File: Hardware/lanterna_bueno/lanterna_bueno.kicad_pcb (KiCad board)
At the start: 2 copper layers, 78.8 x 56.5 mm, 62 parts, among them J1 Conn_01x02_Male, J10 Conn_01x03_Male, J11 Conn_01x03_Male, J2 Conn_01x02_Male, J3 Conn_01x02_Male, J4 Conn_01x03_Male, J5 Conn_01x03_Male, J6 Conn_01x03_Male, J7 Conn_01x03_Male, J8 Conn_01x03_Male, J9 Conn_01x03_Male, P1 USB_C_Plug_USB2.0, Q1 BC807, Q2 2SK4075, Q3 2SK4075, Q4 2SK4075, Q5 2SK4075, SW1 SW_Push, SW2 SW_Push, SW3 SW_Push, U1 RT9193-33, U2 IR2101, U3 IR2101, U4 STM32F042K6Tx, U5 TP4056

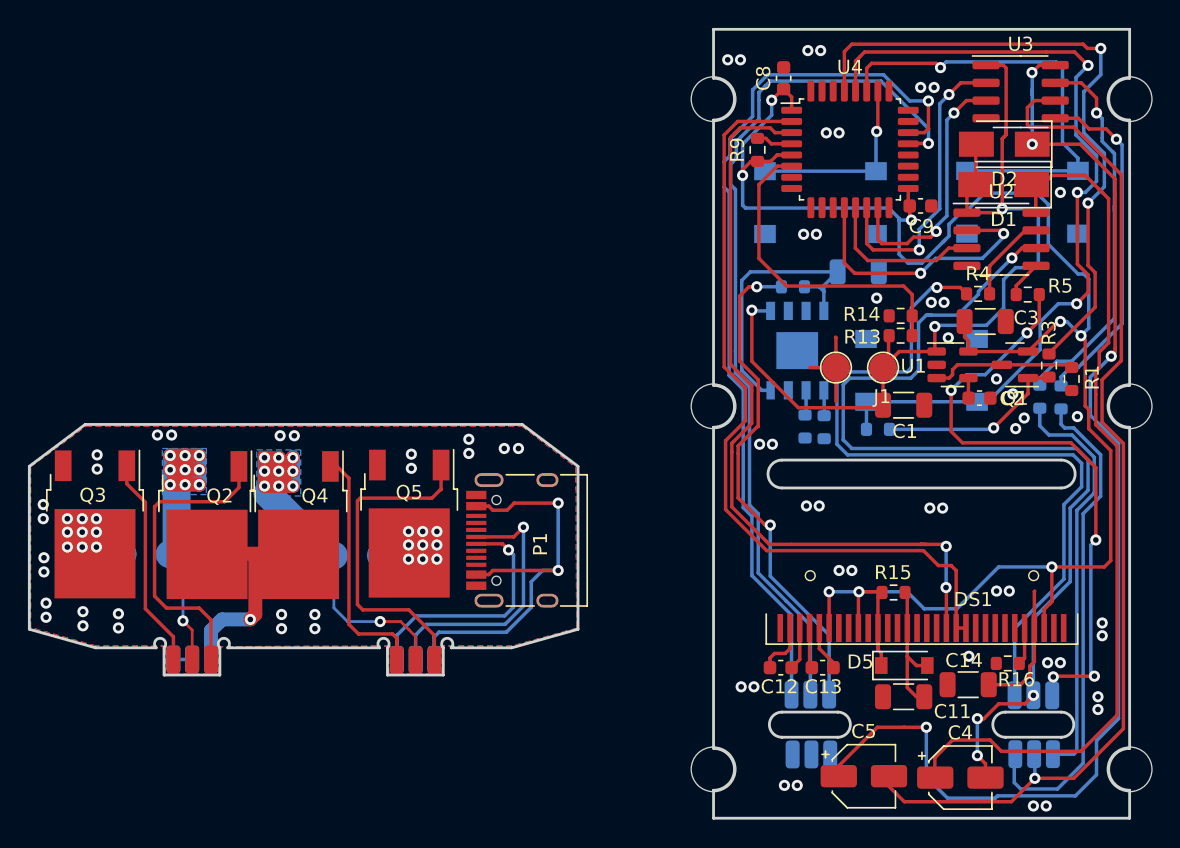
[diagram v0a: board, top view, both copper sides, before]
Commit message: building
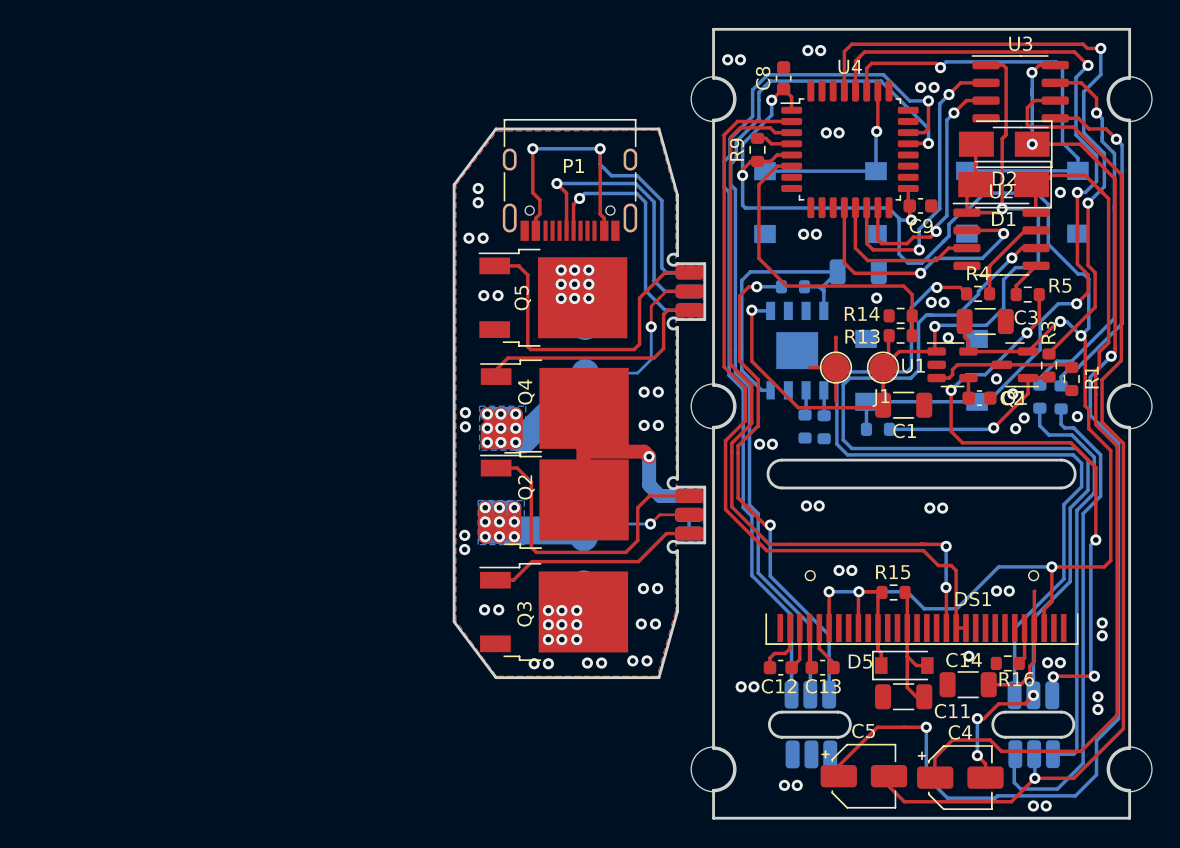
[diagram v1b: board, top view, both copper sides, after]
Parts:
- moved J5 41.6 mm to (136.7, 104.5), turned to -90 degrees
- moved J7 37.1 mm to (136.7, 85.3), turned to 90 degrees
- moved J4 36.5 mm to (136.7, 88.5), turned to -90 degrees
- moved J6 35.0 mm to (131.2, 104.5), turned to -90 degrees
- moved Q3 33.5 mm to (124.3, 109.9), turned to 0 degrees
- moved J2 29.7 mm to (126.4, 104.5), turned to -90 degrees
- moved P1 26.4 mm to (125.4, 78.5), turned to 180 degrees
- moved Q2 25.0 mm to (124.3, 101.8), turned to 0 degrees
- moved J3 22.2 mm to (126.5, 92.8), turned to 90 degrees
- moved Q4 20.2 mm to (124.3, 95.3), turned to 0 degrees
- moved Q5 19.2 mm to (124.2, 87.4), turned to 0 degrees
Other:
- board size 78.8 x 56.5 mm -> 48.4 x 56.5 mm
